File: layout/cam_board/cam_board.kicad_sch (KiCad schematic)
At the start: 0 parts

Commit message: Update layout and schematic
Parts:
- added C1: 2u2F, Capacitor_SMD:C_0504_1310Metric_Pad0.83x1.28mm_HandSolder, symbol Device:C
- added C10, C11: 10pF, Capacitor_SMD:C_0504_1310Metric_Pad0.83x1.28mm_HandSolder, symbol Device:C
- added C2, C3, C4, C7: 100nF, Capacitor_SMD:C_0504_1310Metric_Pad0.83x1.28mm_HandSolder, symbol Device:C
- added C5: 4u7F, Capacitor_SMD:C_0504_1310Metric_Pad0.83x1.28mm_HandSolder, symbol Device:C
- added C6: 1uF, Capacitor_SMD:C_0504_1310Metric_Pad0.83x1.28mm_HandSolder, symbol Device:C
- added C8, C9: 30pF, Capacitor_SMD:C_0504_1310Metric_Pad0.83x1.28mm_HandSolder, symbol Device:C
- added J1: Debug Connector, Connector_PinHeader_1.27mm:PinHeader_1x04_P1.27mm_Vertical, symbol Connector:Conn_01x04_Pin
- added U1: STM32F401CCUx, Package_DFN_QFN:QFN-48-1EP_7x7mm_P0.5mm_EP5.6x5.6mm, symbol MCU_ST_STM32F4:STM32F401CCUx
- added Y1: ECS-80-18-23B-JTN-TR, symbol Device:Crystal_GND2
- added Y2: SC32S-7PF20PPM, symbol Device:Crystal
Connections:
- new net: C1.2, U1.22 (VCAP1)
- new net +3V3: C2.2, C3.2, C4.2, C5.2, C6.2, C7.2, J1.4 (Pin_4), U1.24 (VDD), U1.36 (VDD), U1.48 (VDD), U1.9 (VREF+)
- new net BL: U1.41 (PB5)
- new net CLK: U1.15 (PA5)
- new net CS: U1.14 (PA4)
- new net DC: U1.13 (PA3)
- new net DIN: U1.17 (PA7)
- new net GND: C1.1, C10.1, C11.1, C2.1, C3.1, C4.1, C5.1, C6.1, C7.1, C8.1, C9.1, J1.1 (Pin_1), U1.23 (VSS), U1.35 (VSS), U1.47 (VSS), U1.49 (VSS), U1.8 (VSSA), Y1.2
- new net OSC32_IN: C11.2, U1.3 (PC14), Y2.2
- new net OSC32_OUT: C10.2, U1.4 (PC15), Y2.1
- new net OSC_IN: C9.2, U1.5 (PH0), Y1.3
- new net OSC_OUT: C8.2, U1.6 (PH1), Y1.1
- new net RST: U1.12 (PA2)
- new net SCL: U1.21 (PB10)
- new net SDA: U1.39 (PB3)
- new net STICK_X: U1.18 (PB0)
- new net STICK_Y: U1.19 (PB1)
- new net STICK_Z: U1.20 (PB2)
- new net SWCLK: J1.3 (Pin_3), U1.34 (PA13)
- new net SWDIO: J1.2 (Pin_2), U1.37 (PA14)
- new net USER_BUTTON: U1.10 (PA0)
- new net USER_LED: U1.2 (PC13)
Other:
- note added: "Bypass capacitor for internal LDO"
- note added: "Decoupling for each VDD/VSS pair, p. 56 Datasheet"
- note added: "Decoupling for each VDDA/VSSA pair, p. 56 Datasheet"
- note added: "HSE circuit 2*(CL - Cstray) Capacitors: high quality (5pf to 25pf) ToDo: double check capacitance"
- note added: "LSE circuit ToDo: double check capacitance and crystal"

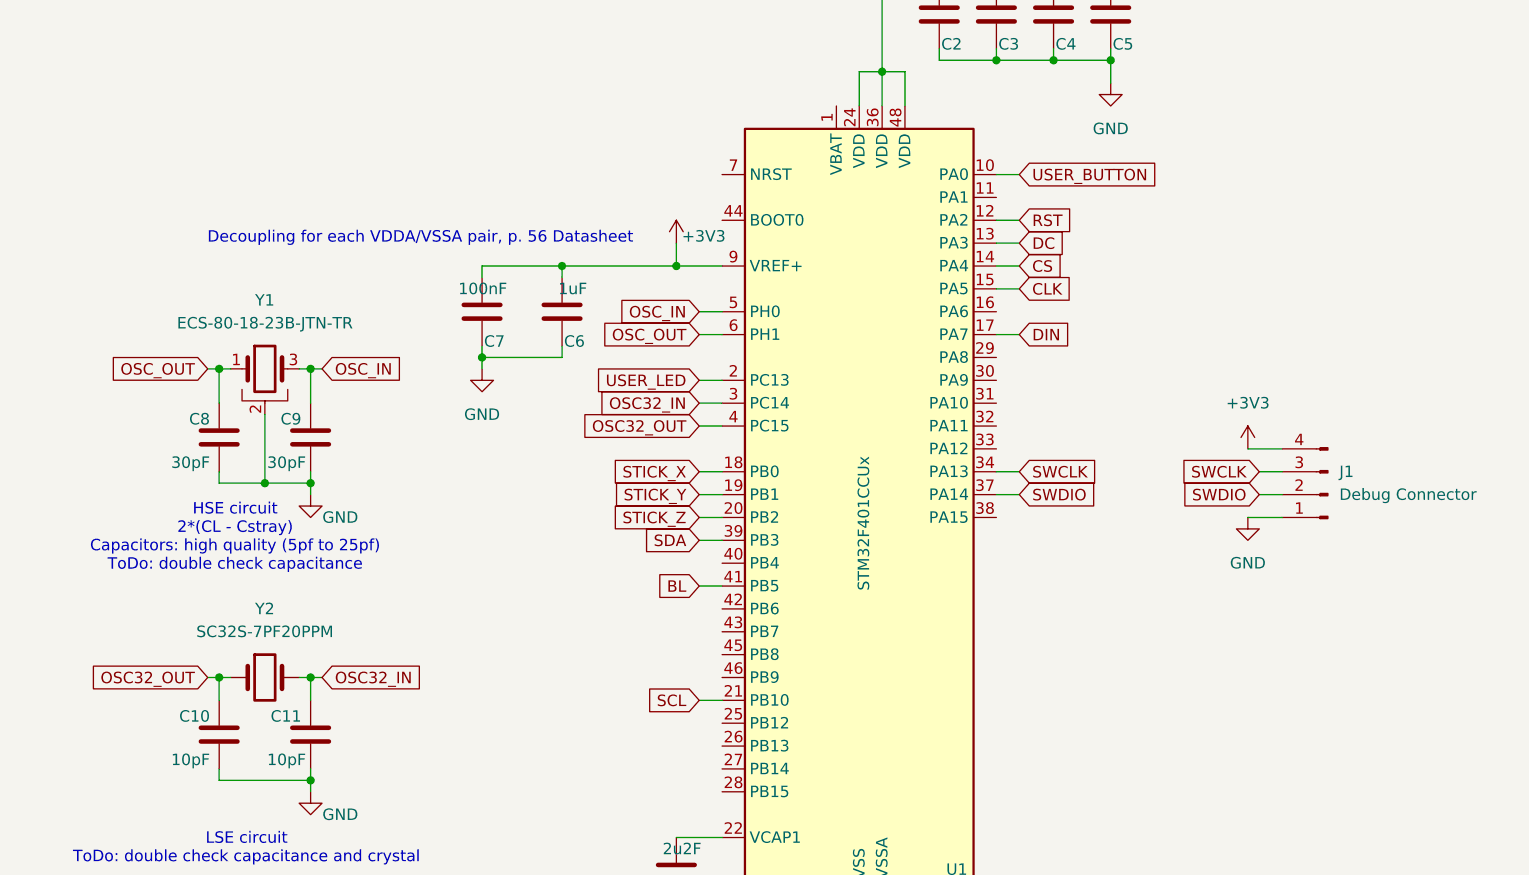
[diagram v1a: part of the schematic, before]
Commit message: Update layout and schematic
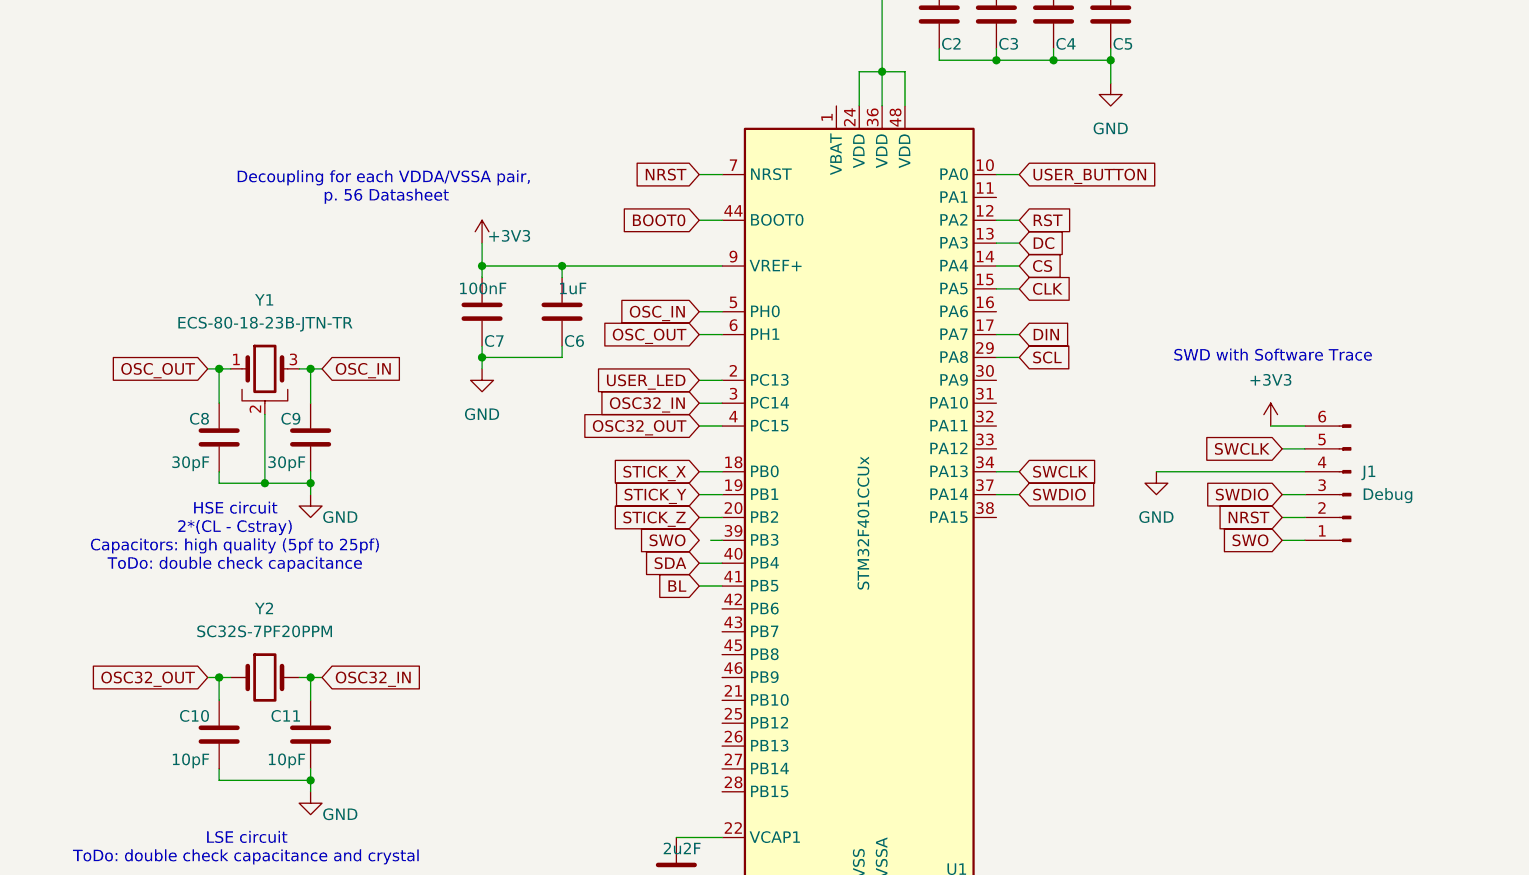
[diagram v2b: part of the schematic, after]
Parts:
- removed J1: Debug Connector, Connector_PinHeader_1.27mm:PinHeader_1x04_P1.27mm_Vertical, symbol Connector:Conn_01x04_Pin
- added J1: Debug, symbol Connector:Conn_01x06_Pin
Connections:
- net +3V3: now also J1.6 (Pin_6)
- net GND: now also J1.4 (Pin_4)
- net SCL: now also U1.29 (PA8); no longer U1.21 (PB10)
- net SDA: now also U1.40 (PB4); no longer U1.39 (PB3)
- net SWCLK: now also J1.5 (Pin_5)
- net SWDIO: now also J1.3 (Pin_3)
- net BOOT0: now reaches U1.44 (BOOT0)
- net NRST: now reaches U1.7 (NRST)
- net NRST: now also J1.2 (Pin_2)
- new net SWO: J1.1 (Pin_1)
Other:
- note added: "SWD with Software Trace"

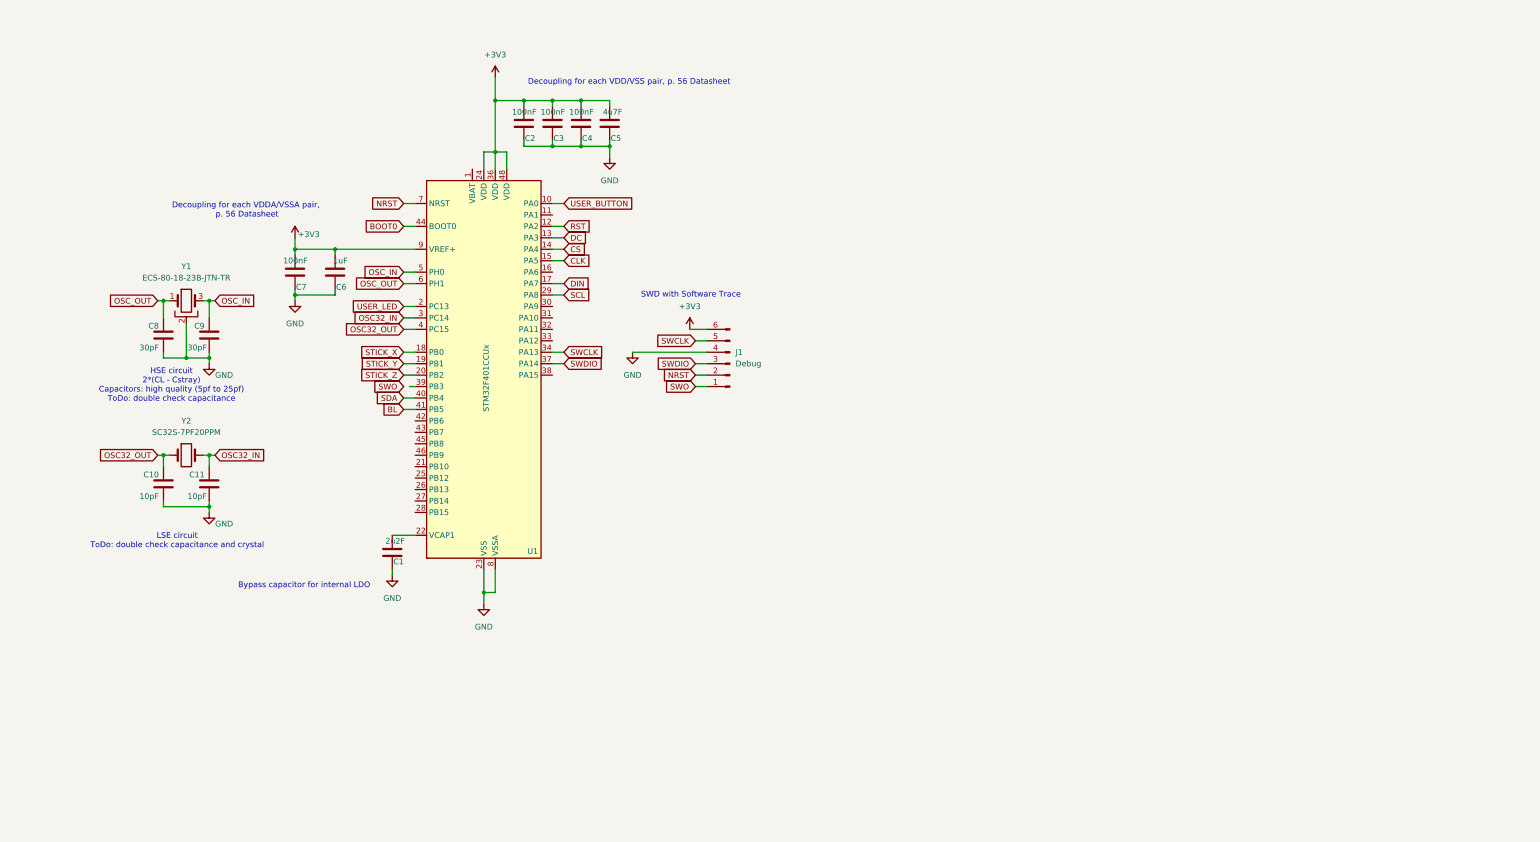
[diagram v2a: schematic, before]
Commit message: Update layout and schematic
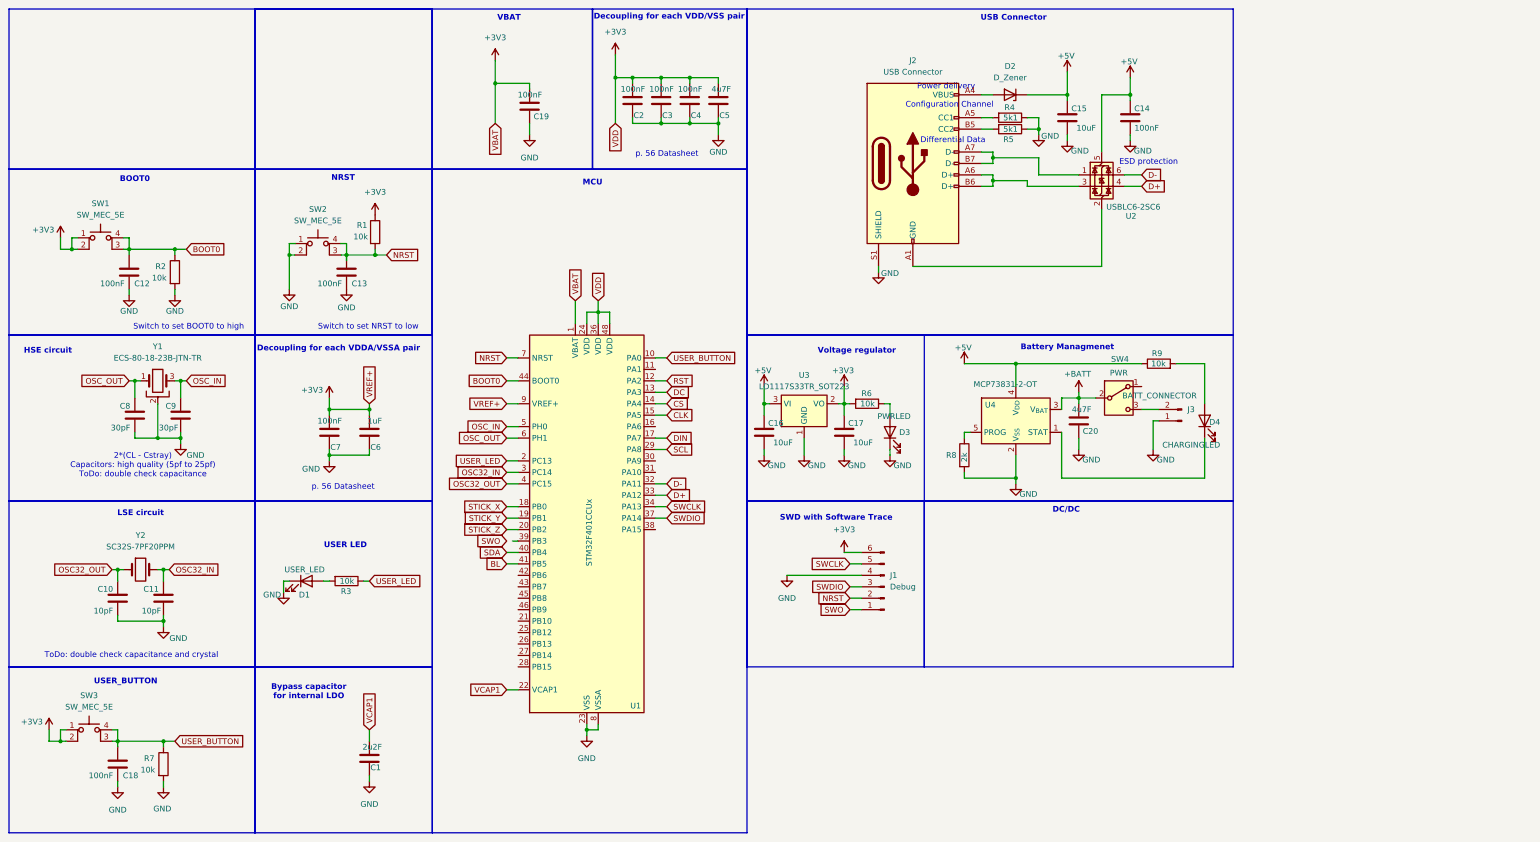
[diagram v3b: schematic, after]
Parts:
- added C12, C13, C14, C18, C19: 100nF, Capacitor_SMD:C_0603_1608Metric_Pad1.08x0.95mm_HandSolder, symbol Device:C
- added C15, C16, C17: 10uF, Capacitor_SMD:C_0603_1608Metric_Pad1.08x0.95mm_HandSolder, symbol Device:C
- added C20: 4u7F, Capacitor_SMD:C_0603_1608Metric_Pad1.08x0.95mm_HandSolder, symbol Device:C
- added D1: USER_LED, LED_SMD:LED_0603_1608Metric_Pad1.05x0.95mm_HandSolder, symbol Device:LED
- added D2: D_Zener, Diode_SMD:D_0201_0603Metric_Pad0.64x0.40mm_HandSolder, symbol Device:D_Zener
- added D3: PWRLED, LED_SMD:LED_0603_1608Metric_Pad1.05x0.95mm_HandSolder, symbol Device:LED
- added D4: CHARGINGLED, LED_SMD:LED_0603_1608Metric_Pad1.05x0.95mm_HandSolder, symbol Device:LED
- added J2: USB Connector, symbol Connector:USB_C_Receptacle_USB2.0_14P
- added J3: BATT_CONNECTOR, symbol Connector:Conn_01x02_Pin
- added R1, R2, R3, R6, R7, R9: 10k, Resistor_SMD:R_0603_1608Metric_Pad0.98x0.95mm_HandSolder, symbol Device:R
- added R4, R5: 5k1, Resistor_SMD:R_0603_1608Metric_Pad0.98x0.95mm_HandSolder, symbol Device:R
- added R8: 2k, Resistor_SMD:R_0603_1608Metric_Pad0.98x0.95mm_HandSolder, symbol Device:R
- added SW1, SW2, SW3: SW_MEC_5E, Button_Switch_SMD:SW_MEC_5GSH9, symbol Switch:SW_MEC_5E
- added SW4: PWR, symbol Switch:SW_SPDT
- added U2: USBLC6-2SC6, Package_TO_SOT_SMD:SOT-23-6_Handsoldering, symbol Power_Protection:USBLC6-2SC6
- added U3: LD1117S33TR_SOT223, Package_TO_SOT_SMD:SOT-223-3_TabPin2, symbol Regulator_Linear:LD1117S33TR_SOT223
- added U4: MCP73831-2-OT, Package_TO_SOT_SMD:SOT-23-5_HandSoldering, symbol Battery_Management:MCP73831-2-OT
- C1, C10, C11, C2, C3, C4, C5, C6, C7, C8, C9: footprint Capacitor_SMD:C_0504_1310Metric_Pad0.83x1.28mm_HandSolder -> Capacitor_SMD:C_0603_1608Metric_Pad1.08x0.95mm_HandSolder
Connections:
- net +3V3: now also U1.1 (VBAT), C17.2, C19.2, R1.1, R6.2, SW1.1, SW1.2, SW3.1, SW3.2, U3.2 (VO)
- net BOOT0: now also C12.2, R2.1, SW1.3 (K), SW1.4 (A)
- net GND: now also C12.1, C13.1, C14.1, C15.1, C16.1, C17.1, C18.1, C19.1, C20.1, D1.1 (K), D3.1 (K), J2.S1 (SHIELD), J3.1 (Pin_1), R2.2, R4.1, R5.1, R7.2, R8.2, SW2.1, SW2.2, U3.1 (GND), U4.2 (V_{SS})
- net NRST: now also C13.2, R1.2, SW2.3 (K), SW2.4 (A)
- net USER_BUTTON: now also C18.2, R7.1, SW3.3 (K), SW3.4 (A)
- net USER_LED: now also R3.1
- net VCAP1: now reaches C1.2, U1.22 (VCAP1)
- net D-: now reaches U1.32 (PA11)
- net D-: now also U2.6 (I/O1)
- net D+: now reaches U1.33 (PA12)
- net D+: now also U2.4 (I/O2)
- new net: J2.B5 (CC2), R5.2
- new net: J2.A5 (CC1), R4.2
- new net: D4.1 (K), U4.1 (STAT)
- new net: D4.2 (A), R9.2
- new net: J3.2 (Pin_2), SW4.3 (C)
- new net: D2.2 (A), J2.A4 (VBUS), J2.A9 (VBUS), J2.B4 (VBUS), J2.B9 (VBUS)
- new net: R8.1, U4.5 (PROG)
- new net: D3.2 (A), R6.1
- new net: J2.A1 (GND), J2.A12 (GND), J2.B1 (GND), J2.B12 (GND), U2.2 (GND)
- new net: J2.A6 (D+), J2.B6 (D+), U2.3 (I/O2)
- new net: J2.A7 (D-), J2.B7 (D-), U2.1 (I/O1)
- new net: D1.2 (A), R3.2
- new net +5V: C14.2, C15.2, C16.2, D2.1 (K), R9.1, U2.5 (VBUS), U3.3 (VI), U4.4 (V_{DD})
- new net +BATT: C20.2, SW4.2 (B), U4.3 (V_{BAT})
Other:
- note added: "2*(CL - Cstray) Capacitors: high quality (5pf to 25pf) ToDo: double check capacitance"
- note added: "BOOT0"
- note added: "Battery Managmenet"
- note added: "Configuration Channel"
- note added: "DC/DC"
- note added: "Decoupling for each VDD/VSS pair"
- note added: "Decoupling for each VDDA/VSSA pair"
- note added: "Differential Data"
- note added: "ESD protection"
- note added: "HSE circuit"
- note added: "LSE circuit"
- note added: "MCU"
- note added: "NRST"
- note added: "Power delivery"
- note added: "Switch to set BOOT0 to high"
- note added: "Switch to set NRST to low"
- note added: "ToDo: double check capacitance and crystal"
- note added: "USB Connector"
- note added: "USER LED"
- note added: "USER_BUTTON"
- note added: "VBAT"
- note added: "Voltage regulator"
- note added: "p. 56 Datasheet"
- note removed: "Decoupling for each VDD/VSS pair, p. 56 Datasheet"
- note removed: "Decoupling for each VDDA/VSSA pair, p. 56 Datasheet"
- note removed: "HSE circuit 2*(CL - Cstray) Capacitors: high quality (5pf to 25pf) ToDo: double check capacitance"
- note removed: "LSE circuit ToDo: double check capacitance and crystal"
- company: (none) -> DonkO
- title: (none) -> CAM-Board
- moved on the sheet: C1, C10, C11, C2, C3, C4, C5, C6, C7, C8, C9, J1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
